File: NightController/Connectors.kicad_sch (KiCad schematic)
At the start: 2 parts, among them J201 Conn_02x20_Odd_Even, J202 Conn_02x20_Odd_Even

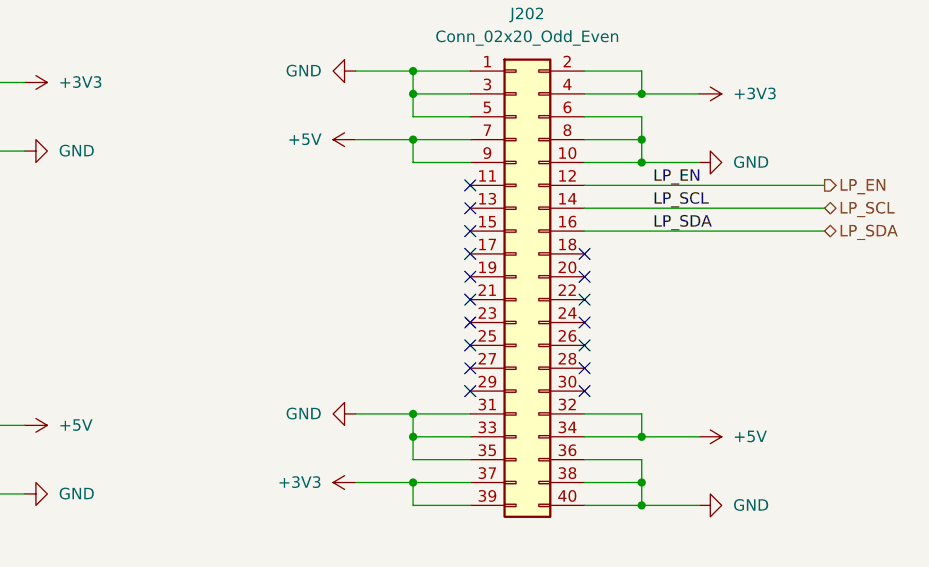
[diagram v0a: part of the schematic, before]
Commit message: Finisched digital one
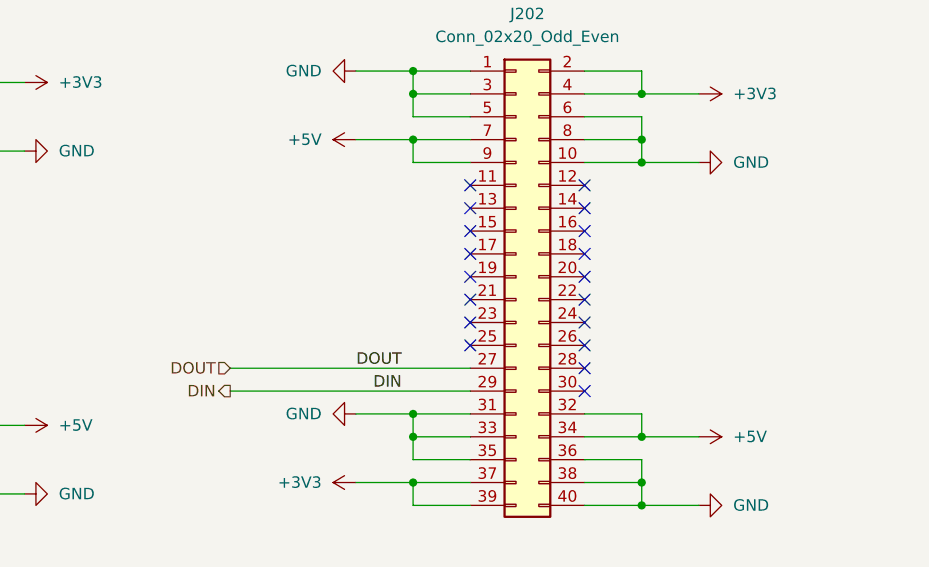
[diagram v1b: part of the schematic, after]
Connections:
- net DOUT: now reaches J202.27 (Pin_27)
- net DIN: now reaches J202.29 (Pin_29)
- net LP_EN: no longer names the net of J202.12 (Pin_12)
- net LP_SCL: no longer names the net of J202.14 (Pin_14)
- net LP_SDA: no longer names the net of J202.16 (Pin_16)
- no-connect marks 37 -> 38
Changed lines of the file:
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@@
+	)
+	(no_connect
+		(at 189.23 81.28)
 	)
 	(no_connect
@@
 	)
 	(no_connect
+		(at 189.23 86.36)
+	)
+	(no_connect
 		(at 189.23 91.44)
 	)
@@
 	)
 	(no_connect
+		(at 189.23 83.82)
+	)
+	(no_connect
 		(at 189.23 104.14)
 	)
@@
 	)
 	(no_connect
-		(at 176.53 101.6)
-	)
-	(no_connect
 		(at 176.53 99.06)
 	)
 	(no_connect
-		(at 176.53 104.14)
-	)
-	(no_connect
 		(at 189.23 93.98)
 	)
@@
 	(wire
 		(pts
-			(xy 189.23 86.36) (xy 215.9 86.36)
-		)
-		(stroke
-			(width 0)
-			(type default)
-		)
-	)
-	(wire
-		(pts
 			(xy 95.25 110.49) (xy 95.25 107.95)
 		)
@@
 	(wire
 		(pts
+			(xy 176.53 101.6) (xy 149.86 101.6)
+		)
+		(stroke
+			(width 0)
+			(type default)
+		)
+	)
+	(wire
+		(pts
 			(xy 176.53 68.58) (xy 170.18 68.58)
 		)
@@
 	(wire
 		(pts
-			(xy 189.23 81.28) (xy 215.9 81.28)
-		)
-		(stroke
-			(width 0)
-			(type default)
-		)
-	)
-	(wire
-		(pts
-			(xy 189.23 83.82) (xy 215.9 83.82)
-		)
-		(stroke
-			(width 0)
-			(type default)
-		)
-	)
-	(wire
-		(pts
 			(xy 120.65 113.03) (xy 120.65 115.57)
 		)
@@
 		(pts
 			(xy 189.23 114.3) (xy 195.58 114.3)
+		)
+		(stroke
+			(width 0)
+			(type default)
+		)
+	)
+	(wire
+		(pts
+			(xy 176.53 104.14) (xy 149.86 104.14)
 		)
 		(stroke
@@
 		)
 	)
-	(label "LP_SDA"
-		(at 196.85 86.36 0)
+	(label "DIN"
+		(at 168.91 104.14 180)
 		(fields_autoplaced yes)
 		(effects
@@
 				(size 1.27 1.27)
 			)
-			(justify left bottom)
-		)
-	)
-	(label "LP_SCL"
-		(at 196.85 83.82 0)
+			(justify right bottom)
+		)
+	)
+	(label "DOUT"
+		(at 168.91 101.6 180)
 		(fields_autoplaced yes)
 		(effects
@@
 				(size 1.27 1.27)
 			)
-			(justify left bottom)
-		)
-	)
-	(label "LP_EN"
-		(at 196.85 81.28 0)
+			(justify right bottom)
+		)
+	)
+	(hierarchical_label "DIN"
+		(shape output)
+		(at 149.86 104.14 180)
 		(fields_autoplaced yes)
 		(effects
@@
 				(size 1.27 1.27)
 			)
-			(justify left bottom)
-		)
-	)
-	(hierarchical_label "LP_SDA"
-		(shape bidirectional)
-		(at 215.9 86.36 0)
+			(justify right)
+		)
+	)
+	(hierarchical_label "DOUT"
+		(shape input)
+		(at 149.86 101.6 180)
 		(fields_autoplaced yes)
 		(effects
@@
 				(size 1.27 1.27)
 			)
-			(justify left)
-		)
-	)
-	(hierarchical_label "LP_SCL"
-		(shape bidirectional)
-		(at 215.9 83.82 0)
-		(fields_autoplaced yes)
-		(effects
-			(font
-				(size 1.27 1.27)
-			)
-			(justify left)
-		)
-	)
-	(hierarchical_label "LP_EN"
-		(shape output)
-		(at 215.9 81.28 0)
-		(fields_autoplaced yes)
-		(effects
-			(font
-				(size 1.27 1.27)
-			)
-			(justify left)
-		)
-	)
+			(justify right)
+		)
+	)
